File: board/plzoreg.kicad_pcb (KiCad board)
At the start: 2 copper layers, 55 parts, among them J1 IN, J2 OUT, J3 Heatsink Earth, Q1 BTA24-600C, U1 HLK-PM03, U2 H11AA1, U3 MOC3023M, U4 PY32F030K1xTx, X1 SWD

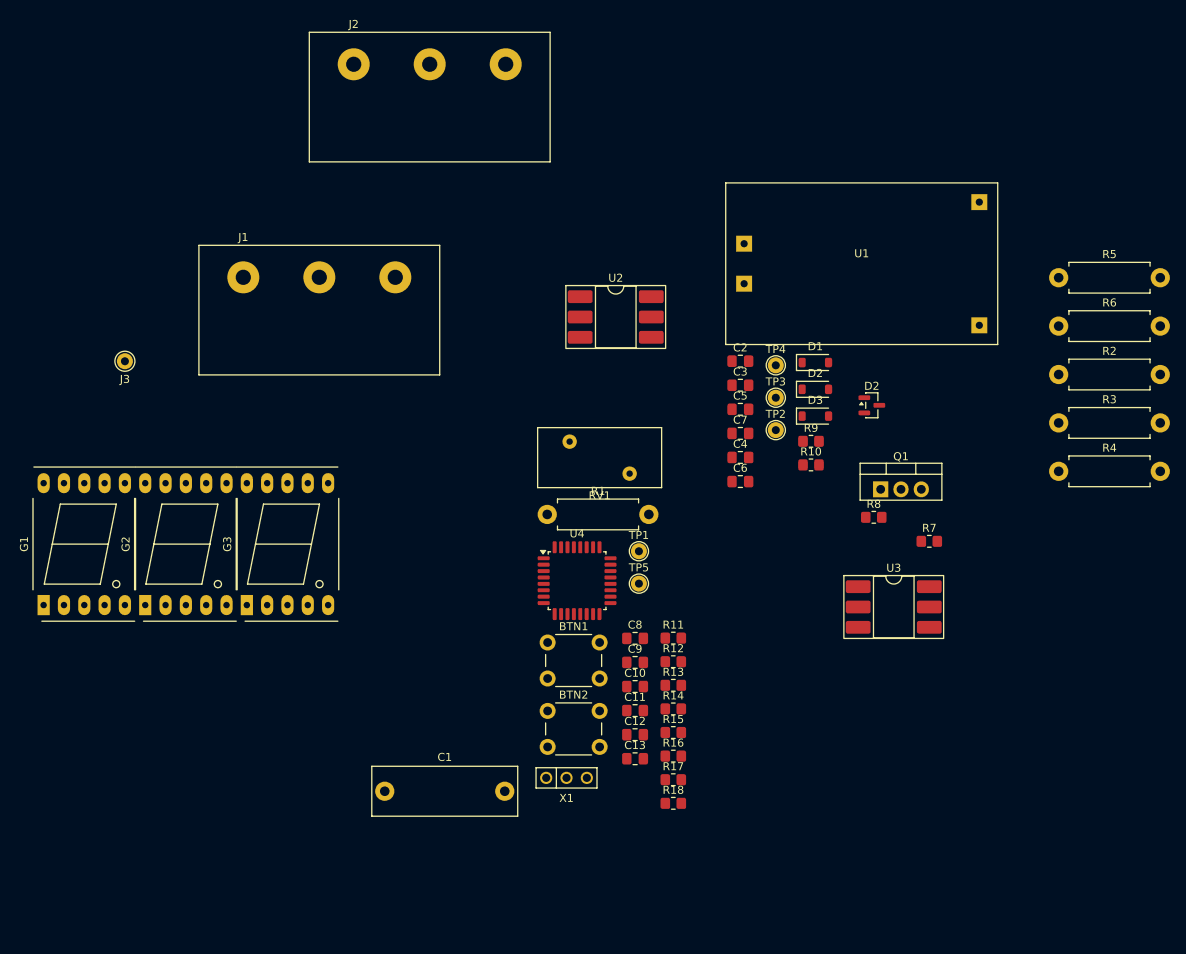
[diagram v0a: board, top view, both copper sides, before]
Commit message: WIP
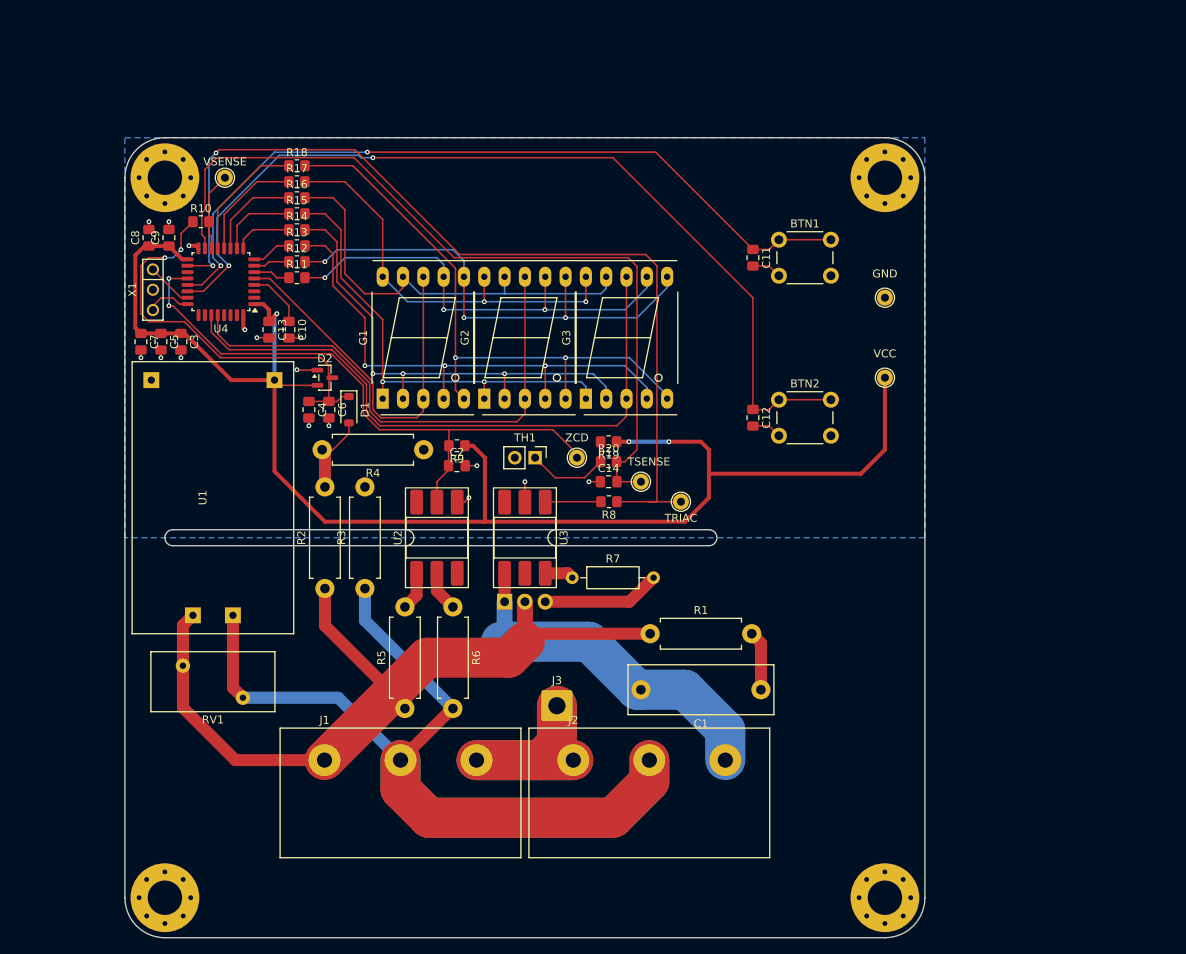
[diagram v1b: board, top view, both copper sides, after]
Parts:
- removed the D2 at (162.5, 82.2)
- removed D3: DSK14, Diode_SMD:D_SOD-123
- added C14: 100n, Capacitor_SMD:C_0805_2012Metric_Pad1.18x1.45mm_HandSolder, F.Cu at (136.7, 93.8)
- added H1: MountingHole, MountingHole:MountingHole_4.3mm_M4_Pad_Via, F.Cu at (81.2, 55.8)
- added H2: MountingHole, MountingHole:MountingHole_4.3mm_M4_Pad_Via, F.Cu at (81.2, 145.8)
- added H3: MountingHole, MountingHole:MountingHole_4.3mm_M4_Pad_Via, F.Cu at (171.2, 145.8)
- added H4: MountingHole, MountingHole:MountingHole_4.3mm_M4_Pad_Via, F.Cu at (171.2, 55.8)
- added R19: 47k 1%, Resistor_SMD:R_0805_2012Metric_Pad1.20x1.40mm_HandSolder, F.Cu at (136.7, 88.8)
- added R20: 1k5, Resistor_SMD:R_0805_2012Metric_Pad1.20x1.40mm_HandSolder, F.Cu at (136.7, 91.3)
- added TH1: 3950, Connector_PinHeader_2.54mm:PinHeader_1x02_P2.54mm_Vertical, F.Cu at (127.5, 90.8)
- added TP6: TSENSE, TestPoint:TestPoint_THTPad_D2.0mm_Drill1.0mm, F.Cu at (140.7, 93.8)
- J3: footprint Connector_Pin:Pin_D1.0mm_L10.0mm -> Connector_Wire:SolderWire-1.5sqmm_1x01_D1.7mm_OD3.9mm
- Q1: moved to B.Cu
- R7: footprint Resistor_SMD:R_0805_2012Metric_Pad1.20x1.40mm_HandSolder -> Resistor_THT:R_Axial_DIN0207_L6.3mm_D2.5mm_P10.16mm_Horizontal
- TP5: value ADC -> VSENSE
- moved R5 97.9 mm to (111.2, 122.2), turned to 90 degrees
- moved R2 95.5 mm to (101.2, 107.2), turned to 90 degrees
- moved R18 92.6 mm to (97.7, 54.3)
- moved J2 91.2 mm to (132.2, 128.6)
- moved R3 89.2 mm to (106.2, 107.2), turned to 90 degrees
- moved R17 88.3 mm to (97.7, 56.3)
- moved U1 86.2 mm to (87.2, 95.8), turned to 90 degrees
- moved R16 84.2 mm to (97.7, 58.3)
- moved R6 83.5 mm to (117.2, 109.5), turned to -90 degrees
- moved R10 82.1 mm to (85.7, 61.3)
- moved R15 80.1 mm to (97.7, 60.3)
- moved X1 80.0 mm to (79.7, 69.8), turned to -90 degrees
- moved R4 79.4 mm to (113.5, 89.8), turned to 180 degrees
- moved C9 78.8 mm to (81.7, 63.3), turned to 90 degrees
- moved C8 78.7 mm to (79.2, 63.3), turned to 90 degrees
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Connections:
- J1 pad 1: /MAIN_PEN -> /MAINS_L_IN
- J1 pad 3: /MAINS_L_IN -> /MAIN_PE
- J2 pad 1: /MAIN_PEN -> /MAIN_PE
- J3 pad 1: /MAIN_PEN -> /MAIN_PE
- R10 pad 2: /ADC -> /VSENSE
- TP5 pad 1: Net-(D1-K) -> /VSENSE
- U4 pad 14: /ADC -> /VSENSE
- U4 pad 15: /ZCD -> /TSENSE
- U4 pad 20: unconnected-(U4-PA10-OSC32IN-Pad20) -> /ZCD
- U4 pad 26: /DISP_CC1 -> unconnected-(U4-PB3-Pad26)
- U4 pad 27: /DISP_CC2 -> /DISP_CC3
- U4 pad 28: /DISP_CC3 -> /DISP_CC2
- U4 pad 5: unconnected-(U4-PF3-Pad5) -> /DISP_CC1
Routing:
- net VCC: track 0.00 -> 186.8 mm, vias 0 -> 3
- net /MAINS_N: track 0.00 -> 144.0 mm
- net /TRIAC: track 0.00 -> 117.6 mm, vias 0 -> 2
- net /BTN2: track 0.00 -> 115.0 mm, vias 0 -> 2
- net /MAINS_L_IN: track 0.00 -> 103.9 mm
- net /TSENSE: track 0.00 -> 102.0 mm
- net /BTN1: track 0.00 -> 98.1 mm, vias 0 -> 2
- net /DISP_CC3: track 0.00 -> 78.8 mm
- net /ZCD: track 0.00 -> 76.6 mm, vias 0 -> 2
- net /DISP_AP: track 0.00 -> 74.8 mm, vias 0 -> 2
- net /DISP_AC: track 0.00 -> 65.6 mm, vias 0 -> 3
- net /DISP_CC2: track 0.00 -> 64.9 mm
- net /DISP_AB: track 0.00 -> 61.6 mm, vias 0 -> 3
- net /DISP_AD: track 0.00 -> 60.5 mm, vias 0 -> 3
- net /DISP_AE: track 0.00 -> 57.9 mm, vias 0 -> 2
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- added copper zone on B.Cu, net GND
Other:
- board outline added: 100 x 100 mm
